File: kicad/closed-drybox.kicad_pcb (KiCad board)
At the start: 2 copper layers, 99.5 x 99.6 mm, 35 parts, among them J1 Power_Jack, M1 Fan, M2 Fan, Q1 AO3400A, Q2 AO3400A, Q3 AO3400A, Q4 AO3400A, Q5 AO3400A, Q6 AO3400A, Q7 AO3400A, U1 AMS1117-3.3, U2 XIAO-ESP32-C6, U3 INA219AxDCN

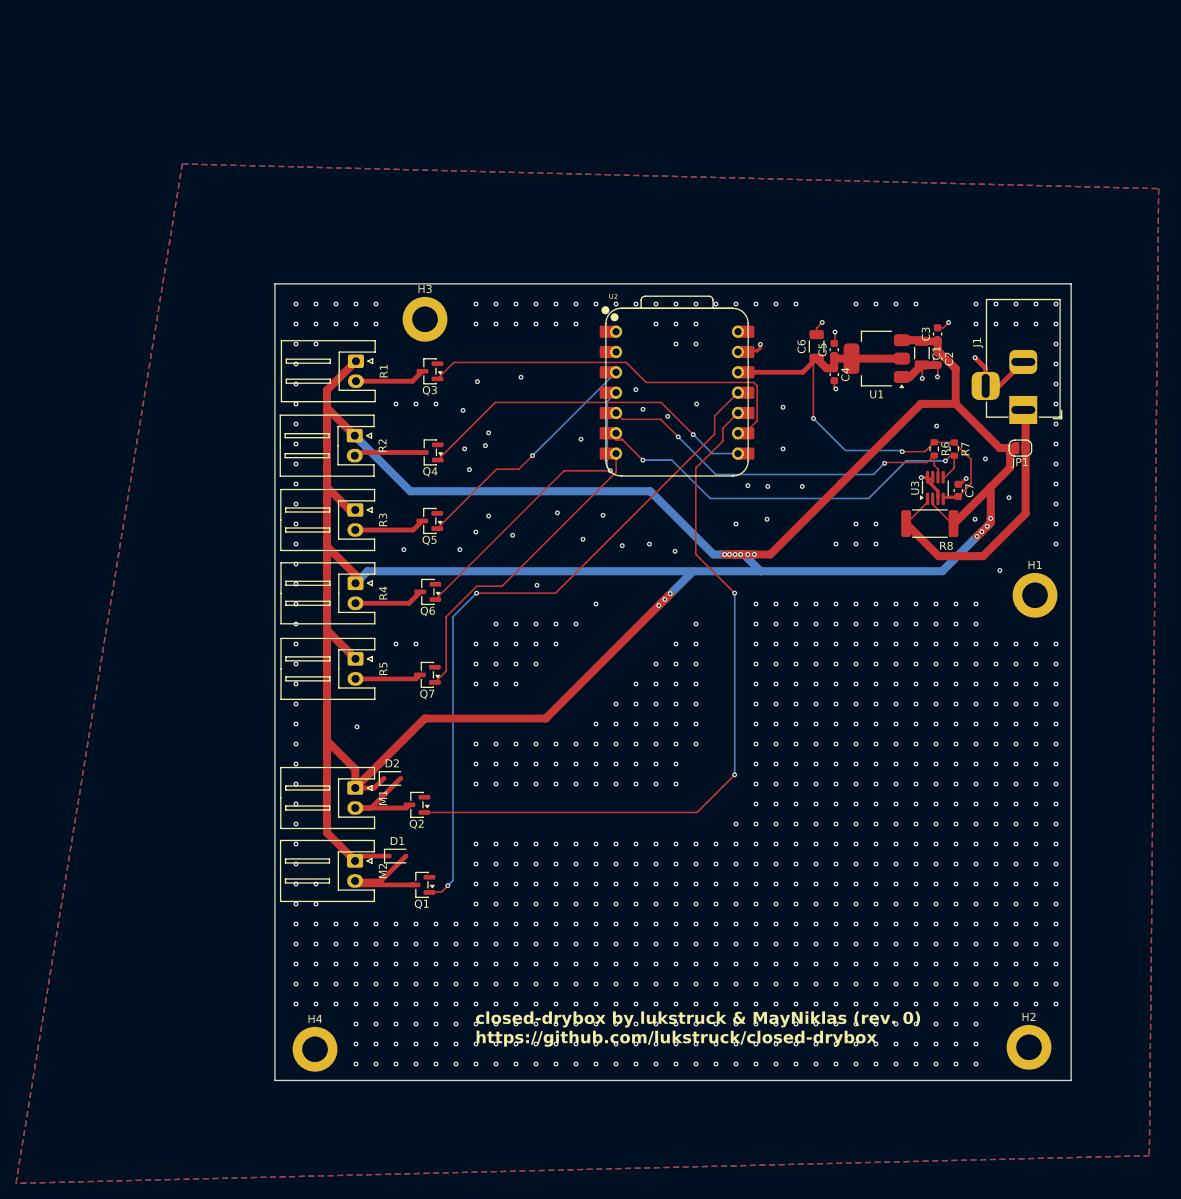
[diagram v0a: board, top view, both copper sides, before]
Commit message: pcb design v0.2
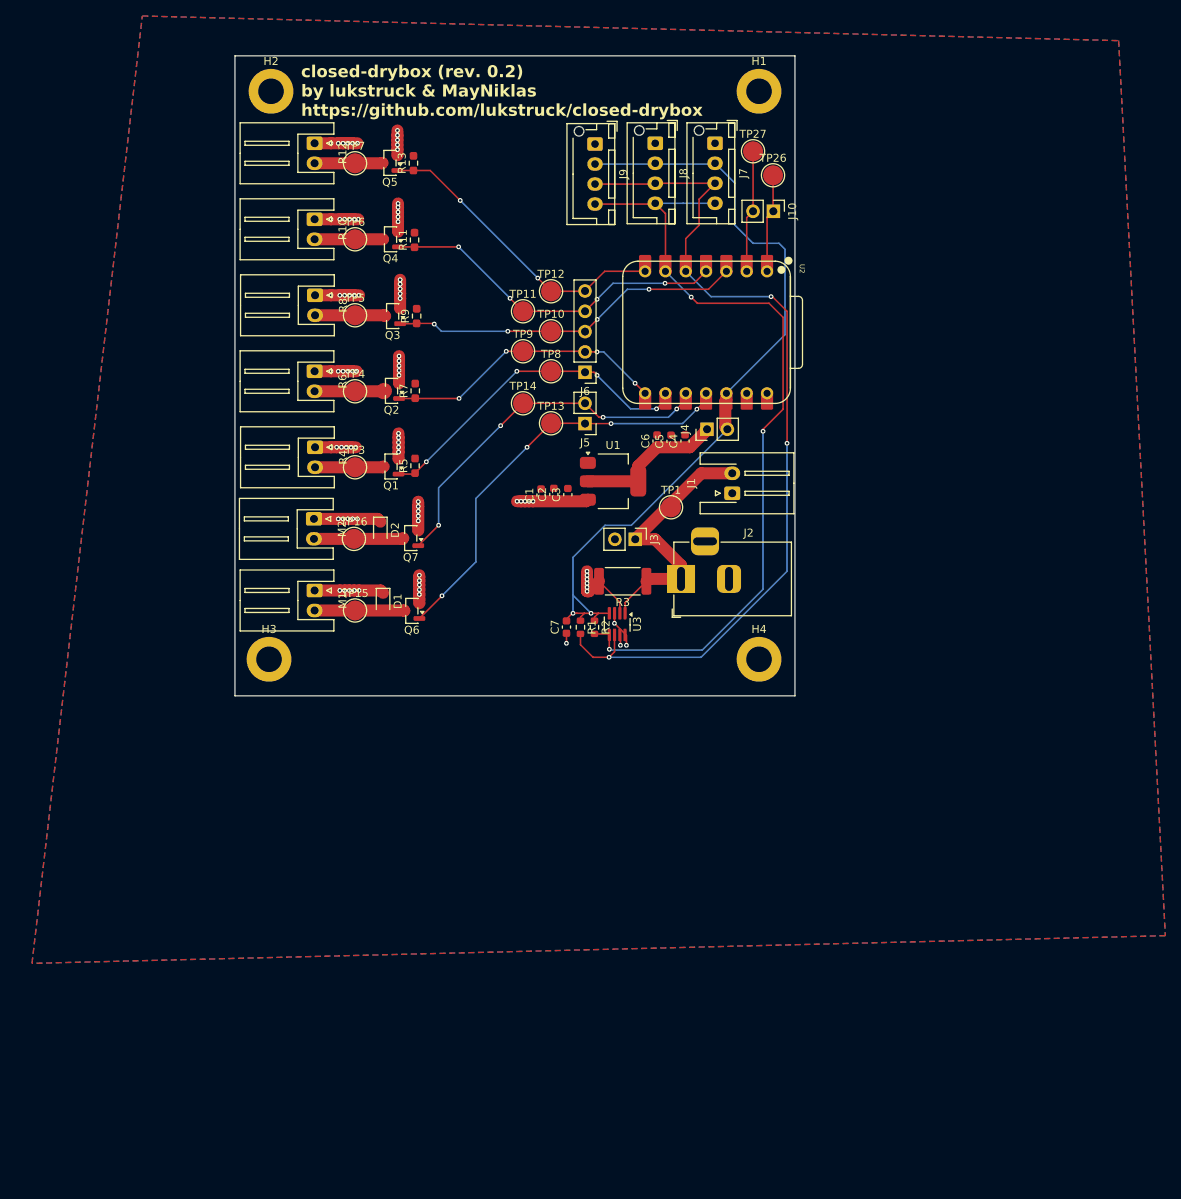
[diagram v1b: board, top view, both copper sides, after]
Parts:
- removed JP1: SolderJumper_2_Open, Jumper:SolderJumper-2_P1.3mm_Open_RoundedPad1.0x1.5mm
- added J10: Conn_01x02_Pin, Connector_PinHeader_2.54mm:PinHeader_1x02_P2.54mm_Vertical, F.Cu at (226.8, 65.5)
- added J2: Power_Jack, Connector_BarrelJack:BarrelJack_Horizontal, F.Cu at (215.2, 111.5)
- added J3: Conn_01x02_Pin, Connector_PinHeader_2.54mm:PinHeader_1x02_P2.54mm_Vertical, F.Cu at (209.5, 106.5)
- added J4: Conn_01x02_Pin, Connector_PinHeader_2.54mm:PinHeader_1x02_P2.54mm_Vertical, F.Cu at (218.5, 92.8)
- added J5: Conn_01x02_Pin, Connector_PinHeader_2.54mm:PinHeader_1x02_P2.54mm_Vertical, F.Cu at (203.2, 92.0)
- added J6: Conn_01x05_Pin, Connector_PinHeader_2.54mm:PinHeader_1x05_P2.54mm_Vertical, F.Cu at (203.2, 85.6)
- added J7: Conn_01x04, Connector_JST:JST_XH_B4B-XH-AM_1x04_P2.50mm_Vertical, F.Cu at (219.5, 57.0)
- added J8: Conn_01x04, Connector_JST:JST_XH_B4B-XH-AM_1x04_P2.50mm_Vertical, F.Cu at (212.0, 57.0)
- added J9: Conn_01x04, Connector_JST:JST_XH_B4B-XH-AM_1x04_P2.50mm_Vertical, F.Cu at (204.5, 57.1)
- added R10: Heater, Connector_JST:JST_XH_S2B-XH-A_1x02_P2.50mm_Horizontal, F.Cu at (169.4, 66.5)
- added R11: 4.7k, Resistor_SMD:R_0603_1608Metric_Pad0.98x0.95mm_HandSolder, F.Cu at (181.9, 69.1)
- added R12: Heater, Connector_JST:JST_XH_S2B-XH-A_1x02_P2.50mm_Horizontal, F.Cu at (169.4, 57.0)
- added R13: 4.7k, Resistor_SMD:R_0603_1608Metric_Pad0.98x0.95mm_HandSolder, F.Cu at (181.8, 59.5)
- added R9: 4.7k, Resistor_SMD:R_0603_1608Metric_Pad0.98x0.95mm_HandSolder, F.Cu at (182.2, 78.6)
- added TP1: TestPoint, TestPoint:TestPoint_Pad_D2.5mm, F.Cu at (214.0, 102.5)
- added TP10: TestPoint, TestPoint:TestPoint_Pad_D2.5mm, F.Cu at (199.0, 80.5)
- added TP11: TestPoint, TestPoint:TestPoint_Pad_D2.5mm, F.Cu at (195.5, 78.0)
- added TP12: TestPoint, TestPoint:TestPoint_Pad_D2.5mm, F.Cu at (199.0, 75.5)
- added TP13: TestPoint, TestPoint:TestPoint_Pad_D2.5mm, F.Cu at (199.0, 92.0)
- added TP14: TestPoint, TestPoint:TestPoint_Pad_D2.5mm, F.Cu at (195.5, 89.5)
- added TP15: TestPoint, TestPoint:TestPoint_Pad_D2.5mm, F.Cu at (174.5, 115.4)
- added TP16: TestPoint, TestPoint:TestPoint_Pad_D2.5mm, F.Cu at (174.4, 106.5)
- added TP26: TestPoint, TestPoint:TestPoint_Pad_D2.5mm, F.Cu at (226.8, 61.0)
- added TP27: TestPoint, TestPoint:TestPoint_Pad_D2.5mm, F.Cu at (224.2, 58.0)
- added TP3: TestPoint, TestPoint:TestPoint_Pad_D2.5mm, F.Cu at (174.5, 97.5)
- added TP4: TestPoint, TestPoint:TestPoint_Pad_D2.5mm, F.Cu at (174.5, 88.0)
- added TP5: TestPoint, TestPoint:TestPoint_Pad_D2.5mm, F.Cu at (174.5, 78.5)
- added TP6: TestPoint, TestPoint:TestPoint_Pad_D2.5mm, F.Cu at (174.5, 69.0)
- added TP7: TestPoint, TestPoint:TestPoint_Pad_D2.5mm, F.Cu at (174.5, 59.5)
- added TP8: TestPoint, TestPoint:TestPoint_Pad_D2.5mm, F.Cu at (199.0, 85.5)
- added TP9: TestPoint, TestPoint:TestPoint_Pad_D2.5mm, F.Cu at (195.5, 83.0)
- C1, C6: footprint Capacitor_SMD:C_1206_3216Metric -> Capacitor_SMD:C_0603_1608Metric
- J1: value Power_Jack -> Conn_01x02; footprint Connector_BarrelJack:BarrelJack_Horizontal -> Connector_JST:JST_XH_S2B-XH-A-1_1x02_P2.50mm_Horizontal
- R1, R2: value Heater -> 10k; footprint Connector_JST:JST_XH_S2B-XH-A_1x02_P2.50mm_Horizontal -> Resistor_SMD:R_0603_1608Metric
- R3: value Heater -> 0.1; footprint Connector_JST:JST_XH_S2B-XH-A_1x02_P2.50mm_Horizontal -> Resistor_SMD:R_2512_6332Metric
- R5: value Heater -> 4.7k; footprint Connector_JST:JST_XH_S2B-XH-A_1x02_P2.50mm_Horizontal -> Resistor_SMD:R_0603_1608Metric_Pad0.98x0.95mm_HandSolder
- R6: value 10k -> Heater; footprint Resistor_SMD:R_0603_1608Metric -> Connector_JST:JST_XH_S2B-XH-A_1x02_P2.50mm_Horizontal
- R7: value 10k -> 4.7k; footprint Resistor_SMD:R_0603_1608Metric -> Resistor_SMD:R_0603_1608Metric_Pad0.98x0.95mm_HandSolder
- R8: value 0.1 -> Heater; footprint Resistor_SMD:R_2512_6332Metric -> Connector_JST:JST_XH_S2B-XH-A_1x02_P2.50mm_Horizontal
- U1: value AMS1117-3.3 -> AMS1117-5.0
- moved H2 152.5 mm to (164.0, 50.5)
- moved R8 82.0 mm to (169.5, 76.0), turned to -90 degrees
- moved R6 78.1 mm to (169.4, 85.5)
- moved H4 73.9 mm to (225.0, 121.5)
- moved H1 71.8 mm to (225.0, 50.5)
- moved R7 67.8 mm to (182.0, 88.0), turned to 90 degrees
- moved Q1 52.4 mm to (179.0, 97.4)
- moved C7 51.9 mm to (200.9, 117.5), turned to 90 degrees
- moved Q2 51.8 mm to (179.1, 88.0)
- moved C2 50.9 mm to (199.3, 100.9), turned to 90 degrees
- moved C1 50.8 mm to (197.8, 101.0), turned to 90 degrees
- moved C3 50.4 mm to (201.1, 100.9)
- moved H3 46.8 mm to (163.8, 121.5)
- moved Q5 45.0 mm to (178.9, 59.5)
- moved R1 43.5 mm to (202.7, 117.5)
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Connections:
- C4 pad 1: +3.3V -> Net-(J4-Pin_1)
- C5 pad 1: +3.3V -> Net-(J4-Pin_1)
- C6 pad 1: +3.3V -> Net-(J4-Pin_1)
- J1 pad 1: /power measurement/IN -> GND
- J1 pad 2: GND -> /power measurement/IN
- M1 pad 2: Net-(D2-A) -> Net-(D1-A)
- M2 pad 2: Net-(D1-A) -> Net-(D2-A)
- Q1 pad 1: /FAN1 -> /HEAT1
- Q1 pad 3: Net-(D1-A) -> Net-(Q1-D)
- Q2 pad 1: /FAN2 -> /HEAT2
- Q2 pad 3: Net-(D2-A) -> Net-(Q2-D)
- Q3 pad 1: /HEAT1 -> /HEAT3
- Q4 pad 1: /HEAT2 -> /HEAT4
- Q5 pad 1: /HEAT3 -> /HEAT5
- Q6 pad 1: /HEAT4 -> /FAN1
- Q6 pad 3: Net-(Q6-D) -> Net-(D1-A)
- Q7 pad 1: /HEAT5 -> /FAN2
- Q7 pad 3: Net-(Q7-D) -> Net-(D2-A)
- R1 pad 1: +12V -> +3.3V
- R1 pad 2: Net-(Q3-D) -> /SDA
- R2 pad 1: +12V -> +3.3V
- R2 pad 2: Net-(Q4-D) -> /SCL
- R3 pad 1: +12V -> /power measurement/IN
- R3 pad 2: Net-(Q5-D) -> +12V
- R4 pad 2: Net-(Q6-D) -> Net-(Q1-D)
- R5 pad 1: +12V -> /HEAT1
- R5 pad 2: Net-(Q7-D) -> GND
- R6 pad 1: +3.3V -> +12V
- R6 pad 2: /SDA -> Net-(Q2-D)
- R7 pad 1: +3.3V -> /HEAT2
- R7 pad 2: /SCL -> GND
- R8 pad 1: /power measurement/IN -> +12V
- R8 pad 2: +12V -> Net-(Q3-D)
- U1 pad 2: +3.3V -> Net-(J4-Pin_1)
- U2 pad 1: unconnected-(U2-GPIO0/A0/D0-Pad1)_1 -> /GPIO0
- U2 pad 14: unconnected-(U2-VBUS-Pad14)_1 -> +5V
- U2 pad 2: unconnected-(U2-GPIO1/A1/D1-Pad2) -> /GPIO1
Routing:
- net +12V: track 383.7 -> 63.9 mm, vias 13 -> 51
- net /SDA: track 47.9 -> 109.5 mm, vias 2 -> 3
- net /SCL: track 53.4 -> 101.9 mm, vias 2 -> 3
- net /FAN2: track 91.0 -> 45.2 mm, vias 2 -> 4
- net +3.3V: track 61.8 -> 100.4 mm
- net /FAN1: track 85.9 -> 51.8 mm, vias 2 -> 4
- net Net-(J4-Pin_1): track 0.00 -> 18.8 mm
- net /GPIO1: track 0.00 -> 14.5 mm
- net /HEAT3: track 31.3 -> 44.3 mm, vias 1 -> 4
- net /GPIO0: track 0.00 -> 11.5 mm
- net Net-(Q2-D): track 0.00 -> 8.70 mm
- net Net-(Q6-D): track 8.69 -> 0.00 mm
- net /HEAT2: track 44.0 -> 35.4 mm, vias 1 -> 4
- net Net-(Q1-D): track 0.00 -> 8.60 mm
- net Net-(Q7-D): track 8.60 -> 0.00 mm
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- added copper zone on In2.Cu, net +12V
- added copper zone on In1.Cu, net GND
- added copper zone on In2.Cu, net GND
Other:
- board size 99.5 x 99.6 mm -> 70 x 80 mm
- copper layers 2 -> 4
- board text added: "${TITLE} (rev. ${REVISION}) by ${COMPANY} ${COMMENT1}"
- board text removed: "${TITLE} by ${COMPANY} (rev. ${REVISION}) ${COMMENT1}"
